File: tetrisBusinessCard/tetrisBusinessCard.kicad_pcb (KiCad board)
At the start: 2 copper layers, 48.7 x 84.5 mm, 502 parts, among them J1 USB_B_Micro, SW1 SW_Push, SW2 SW_Push, SW3 SW_Push, SW4 SW_Push, SW5 SW_Push, SW6 SW_Push, SW7 SW_DPST_x2, SW8 SW_Push, U1 SC091413, U2 W25Q16JVUXIQ, U3 NCP1117-3.3_SOT223, Y1 ABMB-272-T3

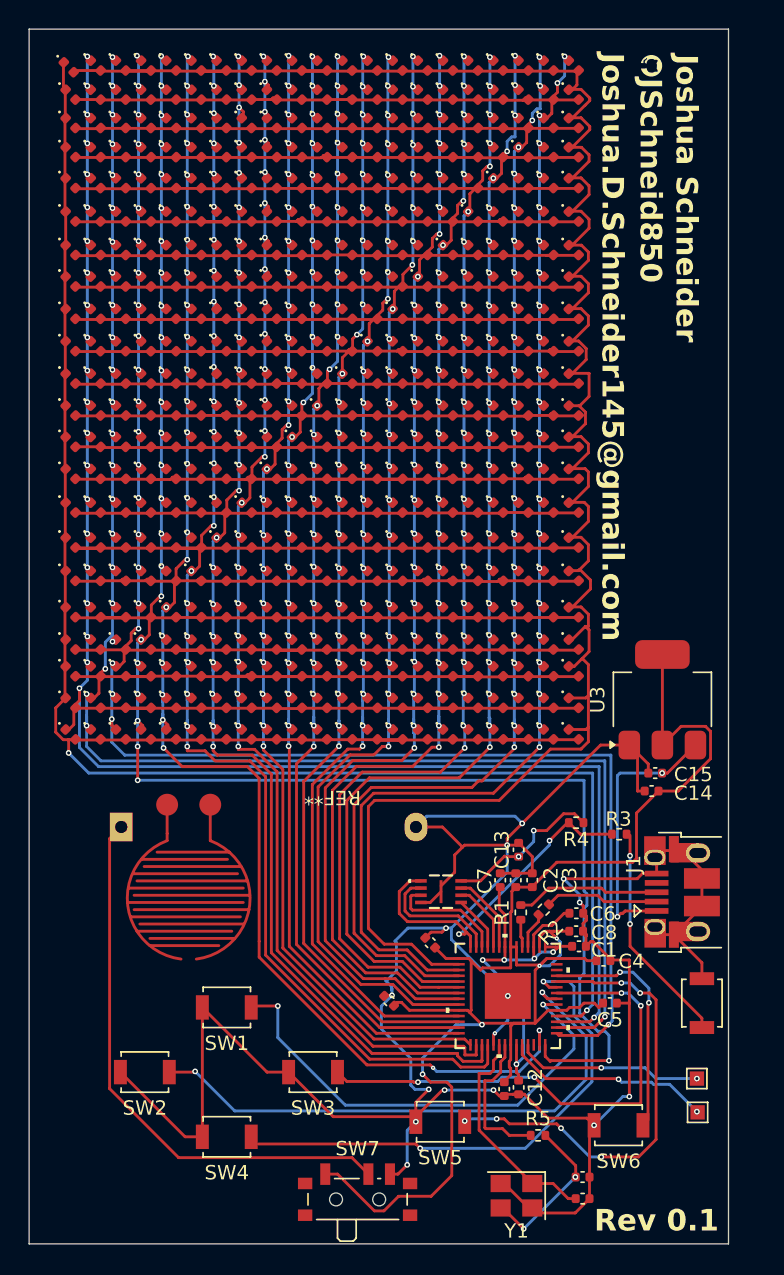
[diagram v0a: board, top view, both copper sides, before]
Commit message: pcb rev0.2
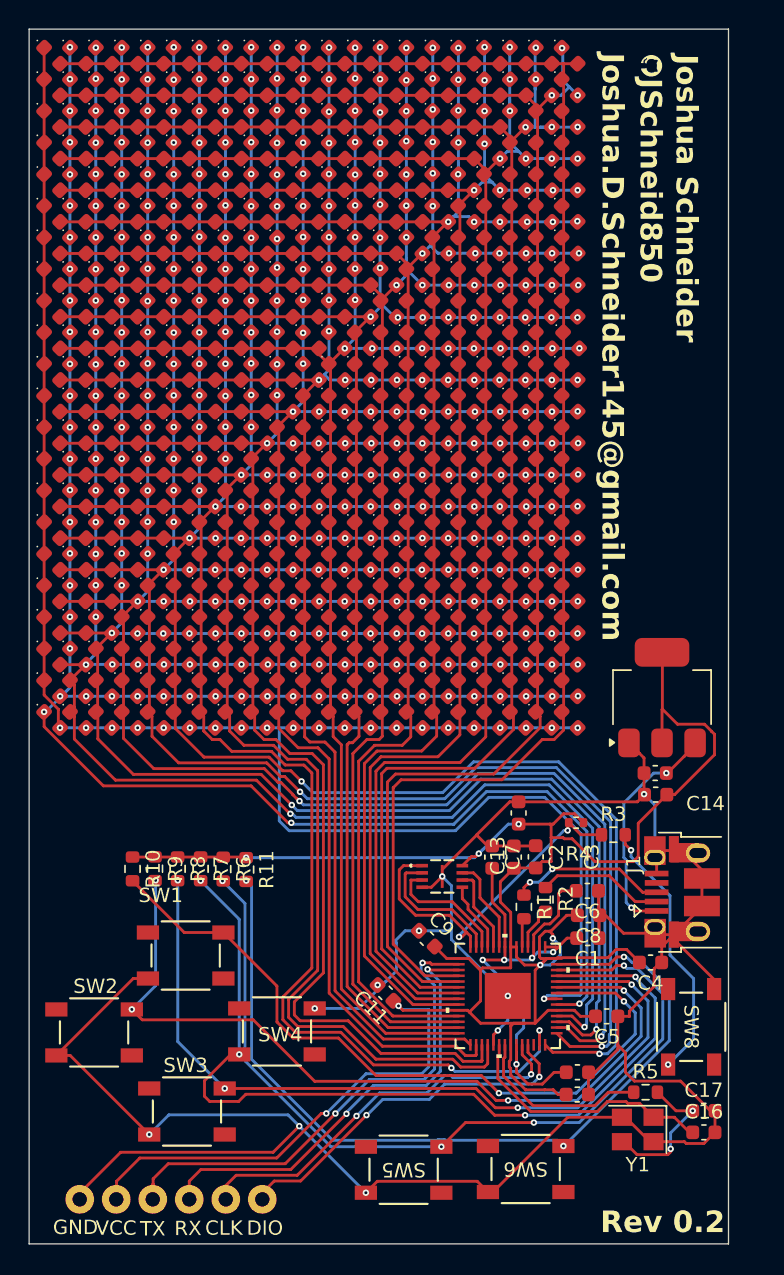
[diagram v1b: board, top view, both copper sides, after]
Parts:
- removed BT1: Battery_Cell, Battery:Battery_Panasonic_CR2032-HFN_Horizontal_CircularHoles
- removed REF** (x2): TestPoint_Pad_1.0x1.0mm, TestPoint:TestPoint_Pad_1.0x1.0mm
- removed REF**: CapacitiveTouchpoint, MyFootprints:CapacitiveTouchpoint
- removed SW7: SW_DPST_x2, Button_Switch_SMD:SW_SPDT_PCM12
- added PogoConnector1: ~, MyFootprints:PogoConnector, F.Cu at (183.7, 104.2)
- added R10: 10kΩ, Resistor_SMD:R_0603_1608Metric, F.Cu at (180.4, 78.2)
- added R11: 10kΩ, Resistor_SMD:R_0603_1608Metric, F.Cu at (188.3, 78.2)
- added R6: 10kΩ, Resistor_SMD:R_0603_1608Metric, F.Cu at (186.7, 78.2)
- added R7: 10kΩ, Resistor_SMD:R_0603_1608Metric, F.Cu at (185.1, 78.2)
- added R8: 10kΩ, Resistor_SMD:R_0603_1608Metric, F.Cu at (183.5, 78.2)
- added R9: 10kΩ, Resistor_SMD:R_0603_1608Metric, F.Cu at (182.0, 78.2)
- C1, C10, C11, C12, C13, C14, C15, C16, C17, C2, C3, C4, C5, C6, C7, C8, C9: footprint Capacitor_SMD:C_0402_1005Metric -> Capacitor_SMD:C_0603_1608Metric
- D1, D10, D100, D101, D102, D103, D104, D105, D106, D107, D108, D109, D11, D110, D111, D112, D113, D114, D115, D116, D117, D118, D119, D12, D120, D121, D122, D123, D124, D125, D126, D127, D128, D129, D13, D130, D131, D132, D133, D134, D135, D136, D137, D138, D139, D14, D140, D141, D142, D143, D144, D145, D146, D147, D148, D149, D15, D150, D151, D152, D153, D154, D155, D156, D157, D158, D159, D16, D160, D161, D162, D163, D164, D165, D166, D167, D168, D169, D17, D170, D171, D172, D173, D174, D175, D176, D177, D178, D179, D18, D180, D181, D182, D183, D184, D185, D186, D187, D188, D189, D19, D190, D191, D192, D193, D194, D195, D196, D197, D198, D199, D2, D20, D200, D201, D202, D203, D204, D205, D206, D207, D208, D209, D21, D210, D211, D212, D213, D214, D215, D216, D217, D218, D219, D22, D220, D221, D222, D223, D224, D225, D226, D227, D228, D229, D23, D230, D231, D232, D233, D234, D235, D236, D237, D238, D239, D24, D240, D241, D242, D243, D244, D245, D246, D247, D248, D249, D25, D250, D251, D252, D253, D254, D255, D256, D257, D258, D259, D26, D260, D261, D262, D263, D264, D265, D266, D267, D268, D269, D27, D270, D271, D272, D273, D274, D275, D276, D277, D278, D279, D28, D280, D281, D282, D283, D284, D285, D286, D287, D288, D289, D29, D290, D291, D292, D293, D294, D295, D296, D297, D298, D299, D3, D30, D300, D301, D302, D303, D304, D305, D306, D307, D308, D309, D31, D310, D311, D312, D313, D314, D315, D316, D317, D318, D319, D32, D320, D321, D322, D323, D324, D325, D326, D327, D328, D329, D33, D330, D331, D332, D333, D334, D335, D336, D337, D338, D339, D34, D340, D341, D342, D343, D344, D345, D346, D347, D348, D349, D35, D350, D351, D352, D353, D354, D355, D356, D357, D358, D359, D36, D360, D361, D362, D363, D364, D365, D366, D367, D368, D369, D37, D370, D371, D372, D373, D374, D375, D376, D377, D378, D379, D38, D380, D381, D382, D383, D384, D385, D386, D387, D388, D389, D39, D390, D391, D392, D393, D394, D395, D396, D397, D398, D399, D4, D40, D400, D401, D402, D403, D404, D405, D406, D407, D408, D409, D41, D410, D411, D412, D413, D414, D415, D416, D417, D418, D419, D42, D420, D421, D422, D423, D424, D425, D426, D427, D428, D429, D43, D430, D431, D432, D433, D434, D435, D436, D437, D438, D439, D44, D440, D441, D442, D443, D444, D445, D446, D447, D448, D449, D45, D450, D451, D452, D453, D454, D455, D456, D457, D458, D459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: footprint LED_SMD:LED_0402_1005Metric -> MyFootprints:LED_0603_1608MetricAdjusted
- R1, R2, R3, R5: footprint Resistor_SMD:R_0402_1005Metric -> Resistor_SMD:R_0603_1608Metric
- SW1, SW2, SW3, SW4, SW5, SW6, SW8: footprint Button_Switch_SMD:SW_SPST_B3U-1000P -> MyFootprints:SW_PTS647SM38SMTR2LFS_CNK
- moved C16 9.61 mm to (220.1, 96.5)
- moved C17 9.61 mm to (220.1, 95.0)
- moved Y1 9.61 mm to (215.5, 96.3)
- moved SW3 9.19 mm to (184.2, 95.0)
- moved SW4 8.12 mm to (190.4, 89.5), turned to 0 degrees
- moved R5 8.06 mm to (216.1, 93.7)
- moved SW6 7.14 mm to (207.7, 99.0)
- moved C10 5.09 mm to (211.3, 93.9), turned to 0 degrees
- moved SW1 4.61 mm to (184.1, 84.2)
- moved SW2 4.48 mm to (177.7, 89.5)
- moved C12 4.22 mm to (211.3, 92.3), turned to 0 degrees
- moved SW5 4.20 mm to (199.2, 99.1)
- moved C4 3.28 mm to (216.4, 84.7)
- moved C13 2.56 mm to (207.2, 74.3)
- moved D399 1.87 mm to (174.8, 61.2)
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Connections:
- net Net-(J1-D+) renamed D+
- net Net-(J1-D-) renamed D-
- C13 pad 1: +3V3 -> BATT +
- R4 pad 1: +3V3 -> BATT +
- SW1 pad 1: BTN_1 -> (no net)
- SW2 pad 1: BTN_2 -> (no net)
- SW3 pad 1: BTN_3 -> (no net)
- SW4 pad 1: BTN_4 -> (no net)
- SW5 pad 1: BTN_5 -> (no net)
- SW6 pad 1: BTN_6 -> (no net)
- SW8 pad 2: Net-(R3-Pad2) -> (no net)
- U1 pad 11: CHRLY_9 -> CHRLY_7
- U1 pad 12: CHRLY_10 -> CHRLY_8
- U1 pad 13: CHRLY_11 -> CHRLY_9
- U1 pad 14: CHRLY_12 -> CHRLY_10
- U1 pad 15: CHRLY_13 -> CHRLY_11
- U1 pad 16: CHRLY_14 -> CHRLY_12
- U1 pad 17: CHRLY_15 -> CHRLY_13
- U1 pad 18: CHRLY_16 -> CHRLY_14
- U1 pad 2: CHRLY_1 -> TX
- U1 pad 24: unconnected-(U1-SWCLK-Pad24) -> SWCLK
- U1 pad 25: unconnected-(U1-SWDIO-Pad25) -> SWDIO
- U1 pad 27: CHRLY_17 -> CHRLY_15
- U1 pad 28: CHRLY_18 -> CHRLY_16
- U1 pad 29: CHRLY_19 -> CHRLY_17
- U1 pad 3: CHRLY_2 -> RX
- U1 pad 30: CHRLY_20 -> CHRLY_18
- U1 pad 31: CHRLY_21 -> CHRLY_19
- U1 pad 32: CHRLY_22 -> CHRLY_20
- U1 pad 34: BTN_1 -> CHRLY_21
- U1 pad 35: BTN_2 -> CHRLY_22
- U1 pad 36: BTN_3 -> BTN_1
- U1 pad 37: BTN_4 -> BTN_2
- U1 pad 38: BTN_5 -> BTN_3
- U1 pad 39: BTN_6 -> BTN_4
- U1 pad 4: CHRLY_3 -> CHRLY_1
- U1 pad 40: unconnected-(U1-GPIO28/ADC2-Pad40) -> BTN_5
- U1 pad 41: unconnected-(U1-GPIO29/ADC3-Pad41) -> BTN_6
- U1 pad 5: CHRLY_4 -> CHRLY_2
- U1 pad 6: CHRLY_5 -> CHRLY_3
- U1 pad 7: CHRLY_6 -> CHRLY_4
- U1 pad 8: CHRLY_7 -> CHRLY_5
- U1 pad 9: CHRLY_8 -> CHRLY_6
- U2 pad 8: +3V3 -> BATT +
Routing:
- net BATT +: track 112.6 -> 168.0 mm, vias 4 -> 7
- net BTN_6: track 16.2 -> 59.7 mm, vias 2 -> 3
- net Net-(BT1-+): track 39.0 -> 0.00 mm
- net TX: track 0.00 -> 35.2 mm, vias 0 -> 2
- net CHRLY_1: track 146.5 -> 112.0 mm
- net RX: track 0.00 -> 31.6 mm, vias 0 -> 2
- net SWCLK: track 0.00 -> 27.8 mm, vias 0 -> 2
- net BTN_5: track 32.1 -> 59.3 mm, vias 6 -> 4
- net BTN_4: track 35.7 -> 61.7 mm, vias 2 -> 4
- net SWDIO: track 0.00 -> 25.2 mm, vias 0 -> 2
- net BTN_3: track 35.3 -> 57.3 mm
- net BTN_1: track 33.0 -> 51.8 mm
- net BTN_2: track 39.6 -> 58.0 mm, vias 2 -> 4
- net CHRLY_18: track 156.6 -> 140.7 mm, vias 25 -> 37
- net unconnected-(U1-SWCLK-Pad24): track 14.5 -> 0.00 mm, vias 2 -> 0
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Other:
- board text added: "CLK"
- board text added: "DIO"
- board text added: "GND"
- board text added: "J1"
- board text added: "RX"
- board text added: "Rev 0.2"
- board text added: "TX"
- board text added: "VCC"
- board text removed: "D127"
- board text removed: "D190"
- board text removed: "D2"
- board text removed: "D22"
- board text removed: "D253"
- board text removed: "Rev 0.1"
